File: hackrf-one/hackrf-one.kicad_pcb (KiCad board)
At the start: 4 copper layers, 120 x 75 mm, 431 parts, among them J1 USB-MICRO-B, J10 GND_CLIP, J2 RF-SHIELD-FRAME, J3 RF-SHIELD-COVER, J4 MOUNTING_HOLE, J5 MOUNTING_HOLE, J6 MOUNTING_HOLE, J7 MOUNTING_HOLE, J8 MOUNTING_HOLE, J9 MOUNTING_HOLE, P13 GPO1, P14 XCVR_CLKOUT, P15 INTR, P16 CLKIN, P17 GPO6, P18 OEB, P19 GPO3, P2 CLKOUT, P20 GPIO, P21 REF_IN, P22 I2S, P23 DBGEN, P24 TRST, P25 LPC_ISP, P26 LPC_JTAG, P27 MIXER_SDATA, P28 SD, P29 CPLD_JTAG, P3 GND, P30 BANK2_AUX, P31 MIXER_SCLK, P32 MIXER_ENX, P33 MIXER_RESETX, P34 MIX_BYPASS, P35 !MIX_BYPASS, P37 SCL, P38 SDA, P39 SSP1_SCK, P4 ANTENNA, P40 SSP1_COPI, P41 SSP1_CIPO, P43 RX, P44 HP, P45 LP, P46 TX_MIX_BP, P47 RX_MIX_BP, P48 TX_AMP, P49 RX_AMP, P5 LEDS, P50 AMP_BYPASS, P51 !TX_AMP_PWR, P52 !RX_AMP_PWR, P53 CS_XCVR, P54 CS_AD, P55 TXENABLE, P56 RXENABLE, P57 XTAL2, P58 GCK1, P59 GCK2, P6 GPO4, P60 SGPIO_CLK, P61 DA0, P62 DA7, P63 DD0, P64 DD9, P65 DA4, P66 DD5, P67 RSSI, P68 SPIFI_CS, P69 VREGMODE, P7 GPO2, P70 EN_1V8, P71 ID, P72 GP_CLKIN, P73 P1_2, P74 P1_1, P75 GP_CLKIN, P76 GP_CLKIN, P77 GP_CLKIN, P78 GP_CLKIN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

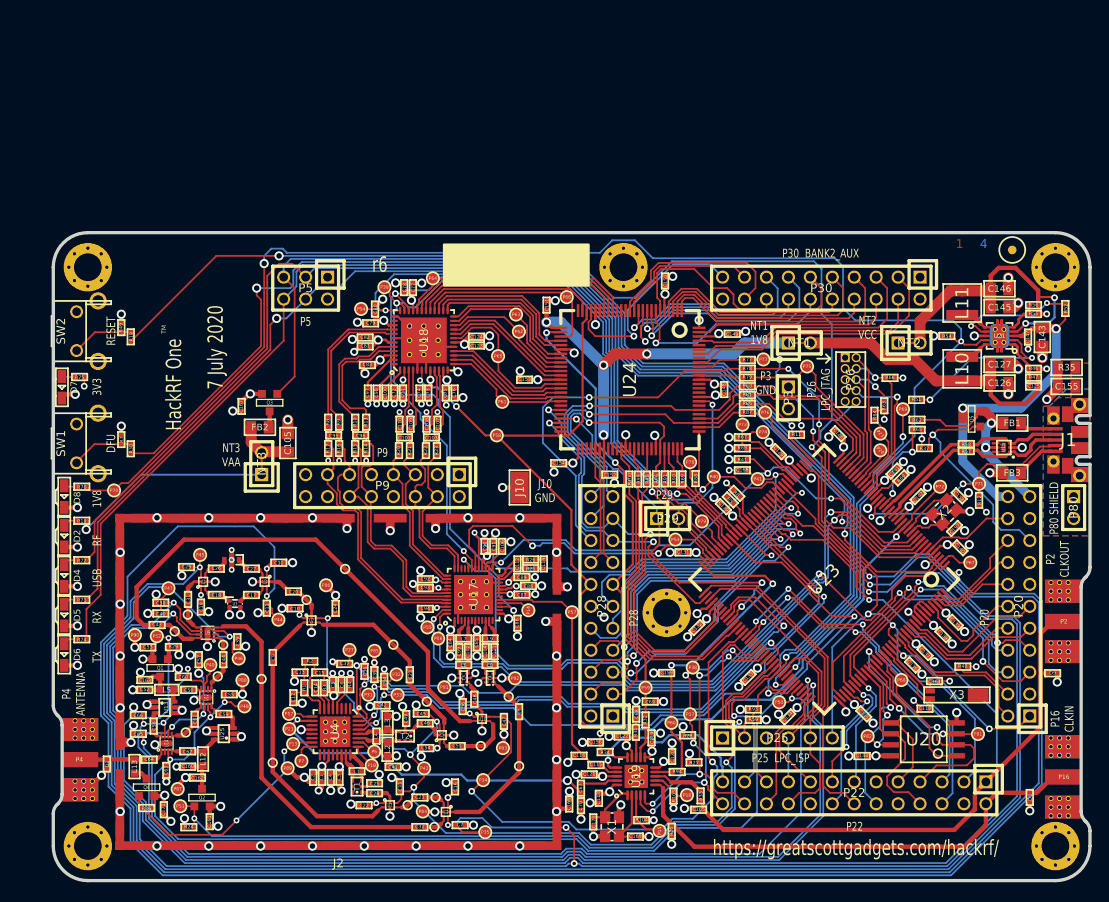
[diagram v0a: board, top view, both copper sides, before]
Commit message: Changes to PCBview
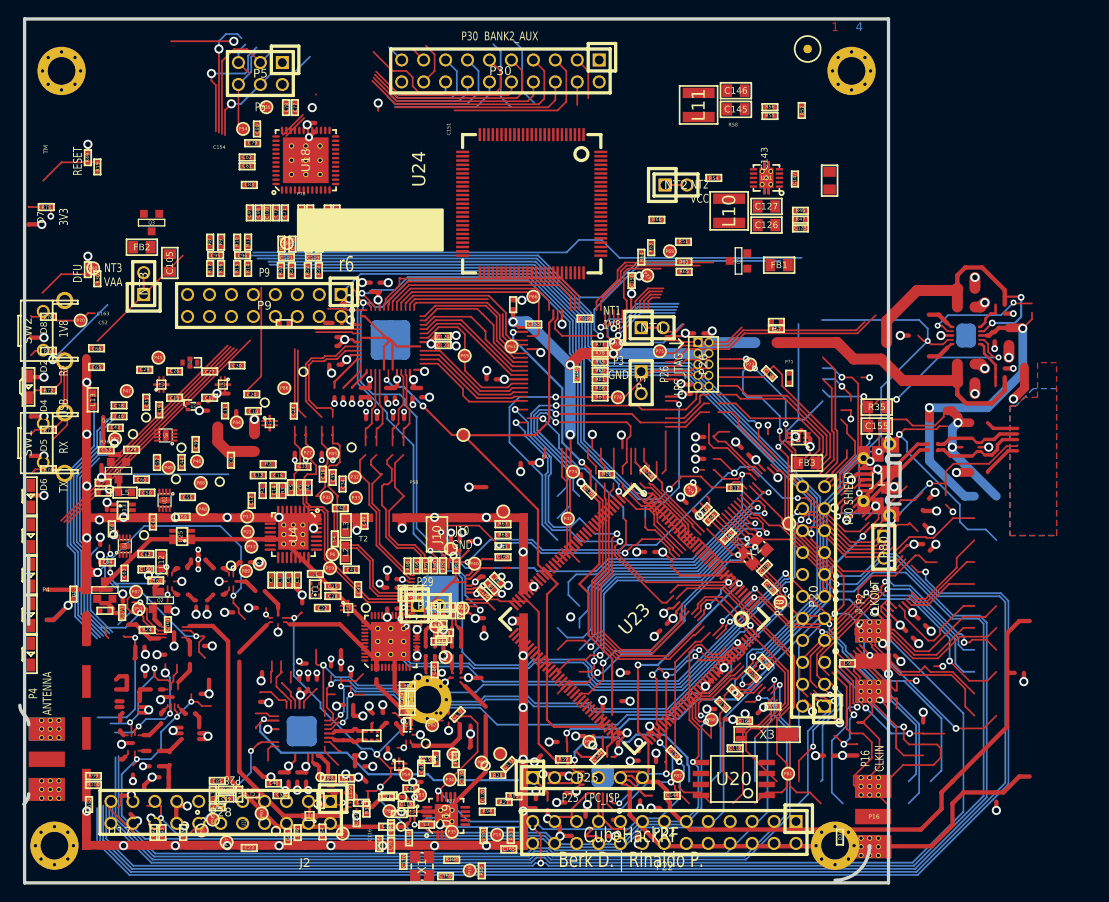
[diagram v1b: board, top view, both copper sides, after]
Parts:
- removed C167: 100nF, hackrf:GSG-0402
- removed J8: MOUNTING_HOLE, hackrf:GSG-HOLE126MIL-COPPER
- moved R99 71.8 mm to (64.6, 162.9), turned to 180 degrees
- moved R100 71.4 mm to (64.6, 163.9), turned to 180 degrees
- moved C152 71.3 mm to (64.1, 166.2), turned to 90 degrees
- moved P28 50.2 mm to (79.4, 167.1), turned to 180 degrees
- moved P57 48.0 mm to (80.1, 170.6), turned to 90 degrees
- moved P30 44.8 mm to (111.8, 81.3)
- moved C92 43.0 mm to (71.6, 169.4), turned to -90 degrees
- moved C65 42.7 mm to (65.0, 115.5)
- moved C66 42.7 mm to (65.0, 113.4)
- moved L13 42.7 mm to (64.6, 119.3)
- moved P90 42.7 mm to (64.6, 104.1)
- moved C93 41.6 mm to (72.6, 169.4), turned to -90 degrees
- moved C146 38.2 mm to (139.0, 83.6)
- moved R52 38.2 mm to (146.6, 85.9)
- moved R56 38.2 mm to (143.0, 85.5)
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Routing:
- net GND: track 592.3 -> 676.4 mm, vias 230 -> 219
- net Net-(FB3-Pad1): track 4.56 -> 80.7 mm
- net MIXER_SDATA: track 72.3 -> 0.00 mm, vias 2 -> 0
- net /mcu/usb/power/ADC0_5: track 11.1 -> 83.3 mm, vias 0 -> 2
- net DA0: track 14.7 -> 74.3 mm
- net /mcu/usb/power/SD_VOLT0: track 39.8 -> 0.00 mm, vias 2 -> 0
- net /mcu/usb/power/XTAL2: track 7.43 -> 47.2 mm, vias 0 -> 2
- net RX_MIX_BP: track 192.3 -> 229.0 mm
- net /mcu/usb/power/VIN: track 39.6 -> 74.0 mm
- net /mcu/usb/power/SD_CLK: track 33.1 -> 0.00 mm, vias 1 -> 0
- net /mcu/usb/power/DP: track 11.3 -> 44.3 mm, vias 0 -> 1
- net /mcu/usb/power/REG_OUT2: track 34.4 -> 2.48 mm
- net LP: track 214.4 -> 185.1 mm
- net TX_MIX_BP: track 215.0 -> 186.3 mm
- net HP: track 210.4 -> 182.8 mm
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- added copper zone on In1.Cu, net GND
- added copper zone on In2.Cu, net VAA
- added copper zone on In2.Cu, net VCC
- removed copper zone on C2, net GND
- removed copper zone on C3, net VAA
- removed copper zone on C3, net VCC
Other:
- board size 120 x 75 mm -> 101.9 x 100 mm
- net class Default removed
- board text added: "CubeHackRF Berk D. | Rinaldo P."
- board text removed: "7 July 2020"
- board text removed: "HackRF One"
- board text removed: "https://greatscottgadgets.com/hackrf/"
